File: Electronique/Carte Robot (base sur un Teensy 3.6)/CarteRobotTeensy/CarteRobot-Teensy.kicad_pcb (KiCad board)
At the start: 2 copper layers, 110 x 100 mm, 25 parts, among them J1 Conn_Bat2, J10 Conn_01x03, J11 Conn_01x05, J12 Conn_01x05, J13 Conn_01x04, J14 Conn_02x04_Counter_Clockwise, J15 Conn_01x04, J18 Adaptateur-Servo-Dynamixel, J2 Conn_Bat1, J22 Conn_01x07, J3 Conn_OnOff, J4 Conn_Aru, J5 Teensy-3.6, J6 Conn_01x04, J7 Conn_01x04, J8 Conn_01x03, J9 Conn_01x03, U1 TSR_1-2450

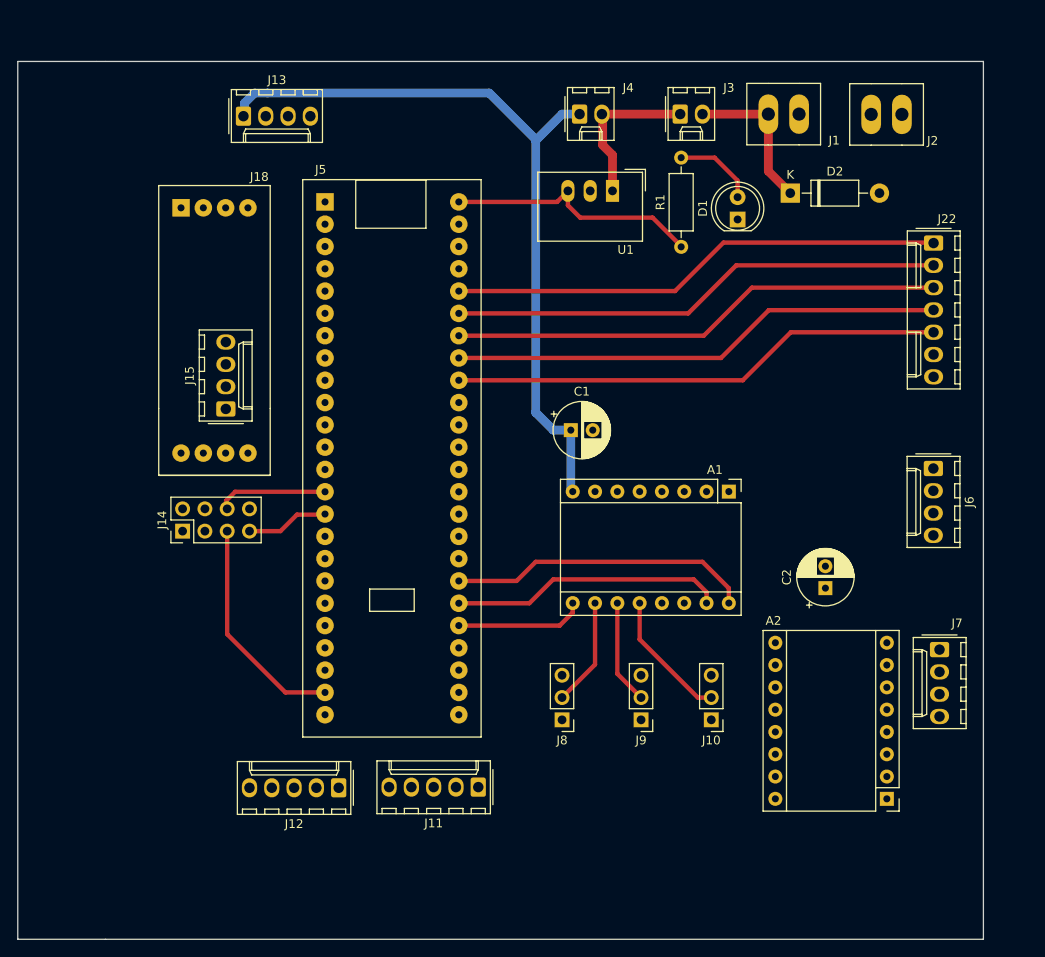
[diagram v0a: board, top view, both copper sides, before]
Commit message: Premiere version pcb
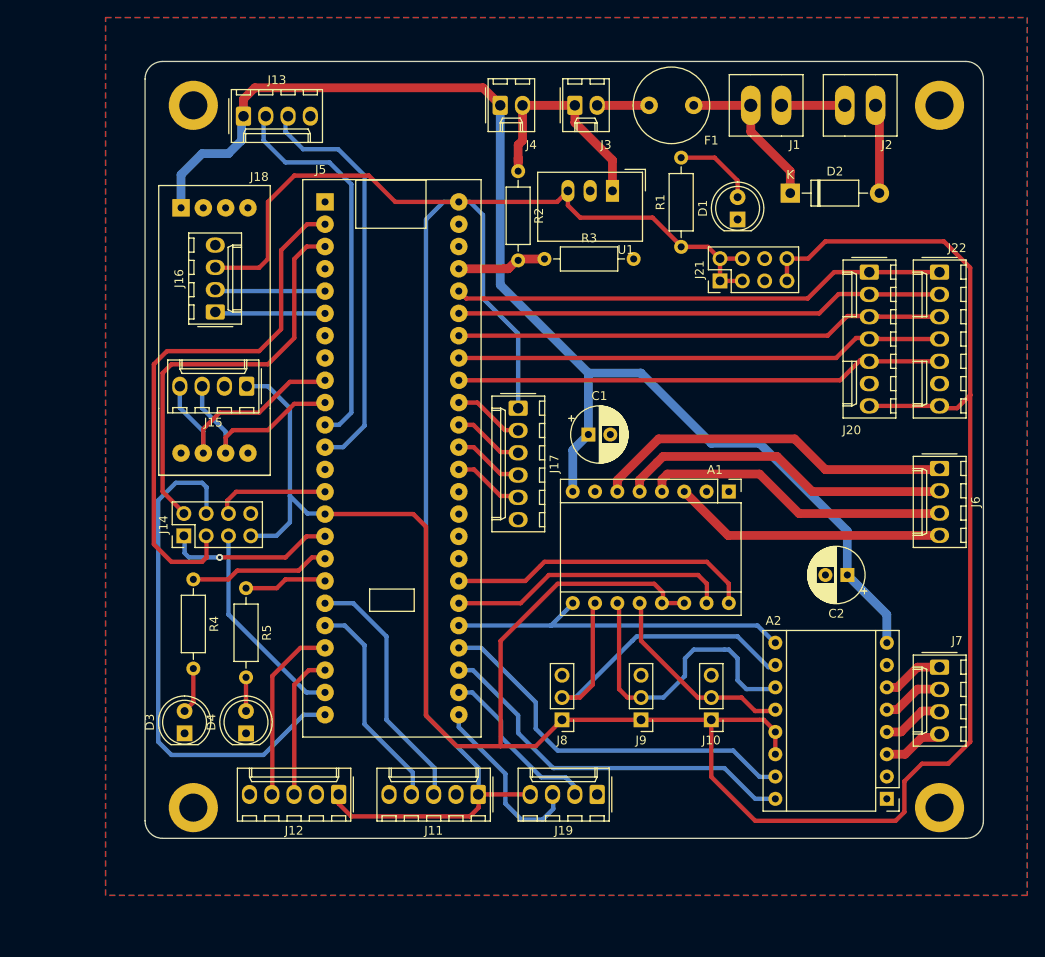
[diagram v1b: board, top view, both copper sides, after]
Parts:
- added D3: LED, LED_THT:LED_D5.0mm_Clear, F.Cu at (59.0, 126.5)
- added D4: LED, LED_THT:LED_D5.0mm_Clear, F.Cu at (66.0, 126.5)
- added F1: Fuse, Fuse:Fuse_Littelfuse_372_D8.50mm, F.Cu at (111.9, 55.0)
- added H1: MountingHole, MountingHole:MountingHole_3.2mm_M3_DIN965_Pad, F.Cu at (145.0, 55.0)
- added H2: MountingHole, MountingHole:MountingHole_3.2mm_M3_DIN965_Pad, F.Cu at (145.0, 135.0)
- added H3: MountingHole, MountingHole:MountingHole_3.2mm_M3_DIN965_Pad, F.Cu at (60.0, 55.0)
- added H4: MountingHole, MountingHole:MountingHole_3.2mm_M3_DIN965_Pad, F.Cu at (60.0, 135.0)
- added J16: Conn_01x04, Connector_Molex:Molex_KK-254_AE-6410-04A_1x04_P2.54mm_Vertical, F.Cu at (62.5, 78.5)
- added J17: Conn_01x06, Connector_Molex:Molex_KK-254_AE-6410-06A_1x06_P2.54mm_Vertical, F.Cu at (97.0, 89.5)
- added J19: Conn_01x04, Connector_Molex:Molex_KK-254_AE-6410-04A_1x04_P2.54mm_Vertical, F.Cu at (106.0, 133.5)
- added J20: Conn_01x07, Connector_Molex:Molex_KK-254_AE-6410-07A_1x07_P2.54mm_Vertical, F.Cu at (137.0, 74.0)
- added J21: Conn_02x04_Counter_Clockwise, Connector_PinHeader_2.54mm:PinHeader_2x04_P2.54mm_Vertical, F.Cu at (120.0, 75.0)
- added R2: 390k, Resistor_THT:R_Axial_DIN0207_L6.3mm_D2.5mm_P10.16mm_Horizontal, F.Cu at (97.0, 62.5)
- added R3: 100k, Resistor_THT:R_Axial_DIN0207_L6.3mm_D2.5mm_P10.16mm_Horizontal, F.Cu at (100.0, 72.5)
- added R4: 500, Resistor_THT:R_Axial_DIN0207_L6.3mm_D2.5mm_P10.16mm_Horizontal, F.Cu at (60.0, 109.0)
- added R5: 500, Resistor_THT:R_Axial_DIN0207_L6.3mm_D2.5mm_P10.16mm_Horizontal, F.Cu at (66.0, 110.0)
- R1: value 100k -> 500
- moved J3 12.0 mm to (103.5, 55.0)
- moved J4 9.10 mm to (95.0, 55.0)
- moved J15 3.51 mm to (66.1, 87.0), turned to 180 degrees
- moved J22 3.38 mm to (145.0, 74.0)
- moved J2 3.17 mm to (134.2, 55.0)
- moved C2 2.92 mm to (134.5, 108.5), turned to 180 degrees
- moved J1 2.24 mm to (123.5, 55.0)
- moved C1 2.06 mm to (105.0, 92.5)
- moved J7 2.00 mm to (145.0, 119.0)
- moved J11 0.84 mm to (92.5, 133.5)
- moved J12 0.76 mm to (76.6, 133.5)
- moved J6 0.70 mm to (145.0, 96.4)
- moved J14 0.55 mm to (58.9, 104.0)
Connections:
- J11 pad 3: (no net) -> /CODG_A
- J11 pad 4: (no net) -> /CODG_B
- J12 pad 3: (no net) -> /CODD_A
- J12 pad 4: (no net) -> /CODD_B
- J18 pad 2: /TX3 -> (no net)
- J18 pad 3: /RX3 -> (no net)
- J18 pad 4: (no net) -> GND
- J18 pad 5: (no net) -> GND
- J18 pad 6: (no net) -> /RX3
- J18 pad 7: (no net) -> /TX3
- J3 pad 2: Net-(D2-Pad1) -> Net-(F1-Pad1)
- J5 pad 17: (no net) -> /LED2
- J5 pad 18: (no net) -> /LED3
- J5 pad 19: (no net) -> /CODG_A
- J5 pad 20: (no net) -> /CODG_B
- J5 pad 21: (no net) -> /CODD_B
- J5 pad 22: (no net) -> /CODD_A
- J5 pad 25: (no net) -> /TX5
- J5 pad 26: (no net) -> /RX5
- J5 pad 27: /STEP_G -> /DIR_G
- J5 pad 28: /DIR_G -> /STEP_G
- J5 pad 36: (no net) -> /14
- J5 pad 37: (no net) -> /15
- J5 pad 38: (no net) -> /16
- J5 pad 39: (no net) -> /17
- J5 pad 45: (no net) -> /Vbat
- J5 pad 5: (no net) -> /CAN0TX
- J5 pad 6: (no net) -> /CAN0RX
- J6 pad 1: Net-(A1-Pad3) -> Net-(A1-Pad6)
- J6 pad 2: /A1D -> Net-(A1-Pad5)
- J6 pad 3: Net-(A1-Pad5) -> /A1D
- J6 pad 4: Net-(A1-Pad6) -> Net-(A1-Pad3)
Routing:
- net +3V3: track 9.44 -> 282.3 mm
- net +5V: track 29.5 -> 204.0 mm
- net /MOSI1: track 0.00 -> 61.4 mm
- net /Varu: track 86.7 -> 147.8 mm
- net /SCK1: track 0.00 -> 59.1 mm
- net /MISO1: track 0.00 -> 46.8 mm
- net /TX2: track 0.00 -> 46.6 mm
- net /RX2: track 0.00 -> 44.2 mm
- net /STEP_G: track 0.00 -> 44.1 mm
- net /DIR_G: track 0.00 -> 43.5 mm
- net Net-(A1-Pad6): track 0.00 -> 41.9 mm
- net Net-(A1-Pad5): track 0.00 -> 38.8 mm
- net /A1D: track 0.00 -> 35.6 mm
- net Net-(A1-Pad3): track 0.00 -> 31.7 mm
- net /M0: track 12.3 -> 42.4 mm
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- added copper zone on B.Cu, net GND
- added copper zone on F.Cu, net GND
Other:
- board size 110 x 100 mm -> 95.5 x 88.5 mm
- net class Default: clearance 0.2 -> 0.3; trace_width 0.25 -> 0.4
- rule trace_clearance: 0.2 -> 0.3
- rule trace_min: 0.2 -> 0.4
- rule via_min_size: 0.4 -> 0.6
